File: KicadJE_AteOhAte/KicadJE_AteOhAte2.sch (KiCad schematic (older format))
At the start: 111 parts, among them J201 In_Accent, J202 In Gate, J203 Out Tom, P201 Doepfer_Power_10pin, Q201 MMBT2222A, Q202 MMBT2222A, Q203 MMBT2222A, Q204 MMBT2222A, Q205 MMBT2907A, Q206 MMBT2222A, Q207 MMBT2222A, SW201 Con/Tom, U201 TL072, U202 TL072, U203 TL072

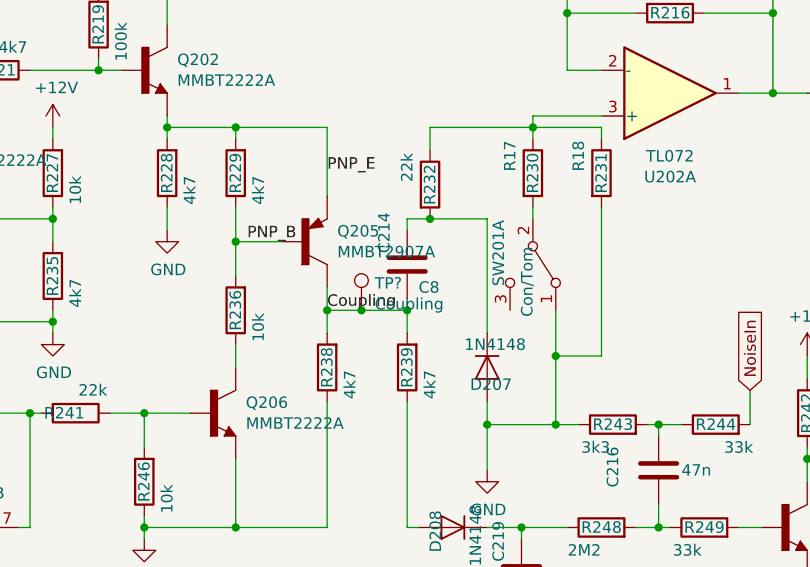
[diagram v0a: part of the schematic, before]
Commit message: Sch
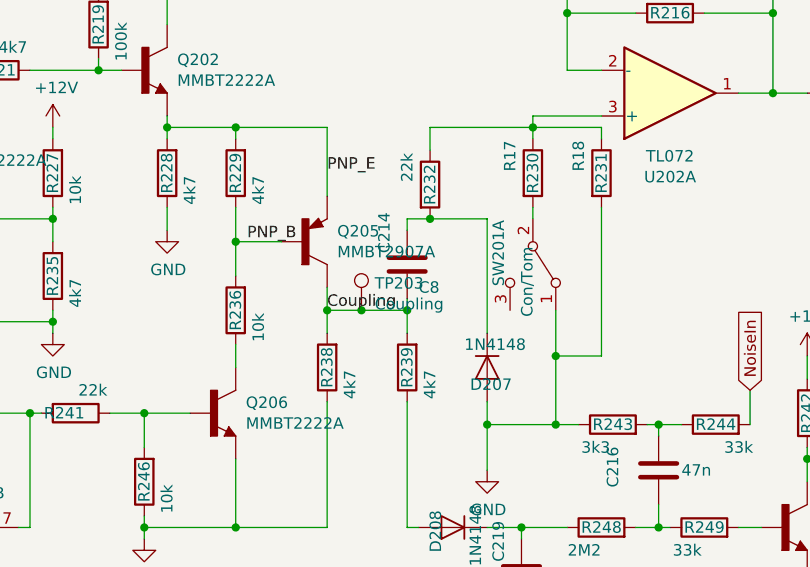
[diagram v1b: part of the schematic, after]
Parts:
- gave numbers to parts that had none: 1
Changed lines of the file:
@@
 	1850 2500 2200 2500
 $Comp
-L Connector:TestPoint TP?
+L Connector:TestPoint TP203
 U 1 1 5DA7BFEF
 P 3800 5950
-F 0 "TP?" H 3858 6068 50  0000 L CNN
+F 0 "TP203" H 3858 6068 50  0000 L CNN
 F 1 "Coupling" H 3858 5977 50  0000 L CNN
 F 2 "TestPoint:TestPoint_Pad_1.5x1.5mm" H 4000 5950 50  0001 C CNN
